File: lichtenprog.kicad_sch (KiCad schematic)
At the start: 54 parts, among them J1 USB_C_Receptacle_USB2.0, J2 IO_OUT, U1 AZ1117-ADJ, U2 MCP6L04x-xSL, U3 USBLC6-2SC6, U4 CP2102N-A01-GQFN28, U5 SN74LVC1T45DBV, U6 SN74LVC1T45DBV

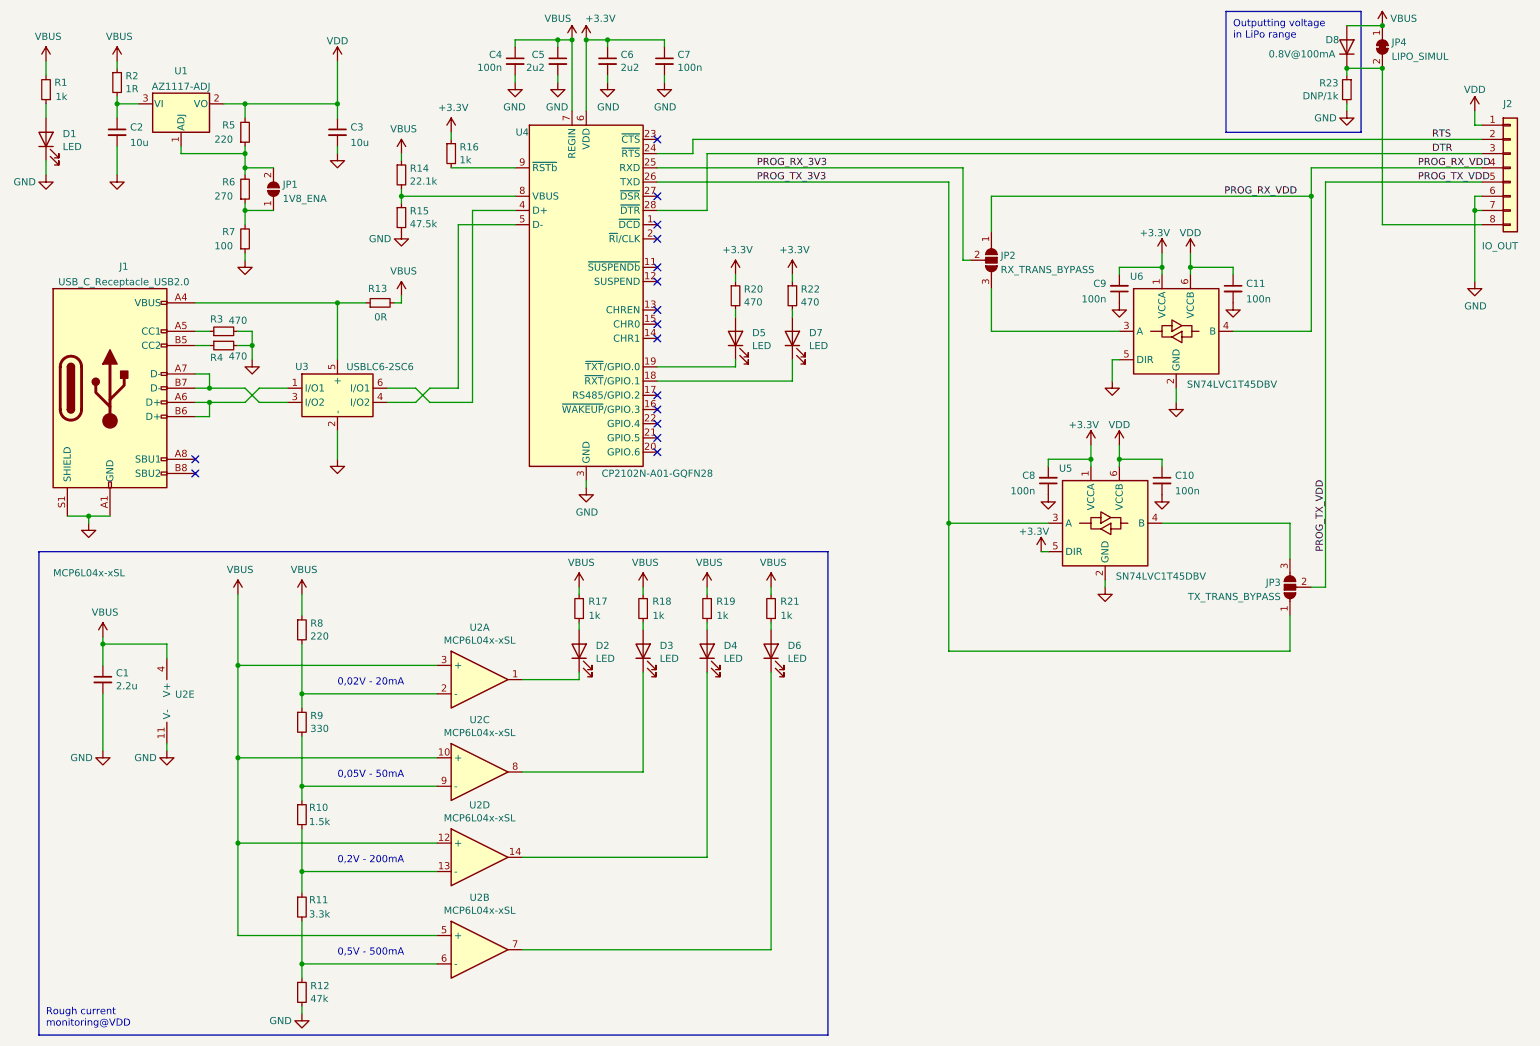
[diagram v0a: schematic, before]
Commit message: idk
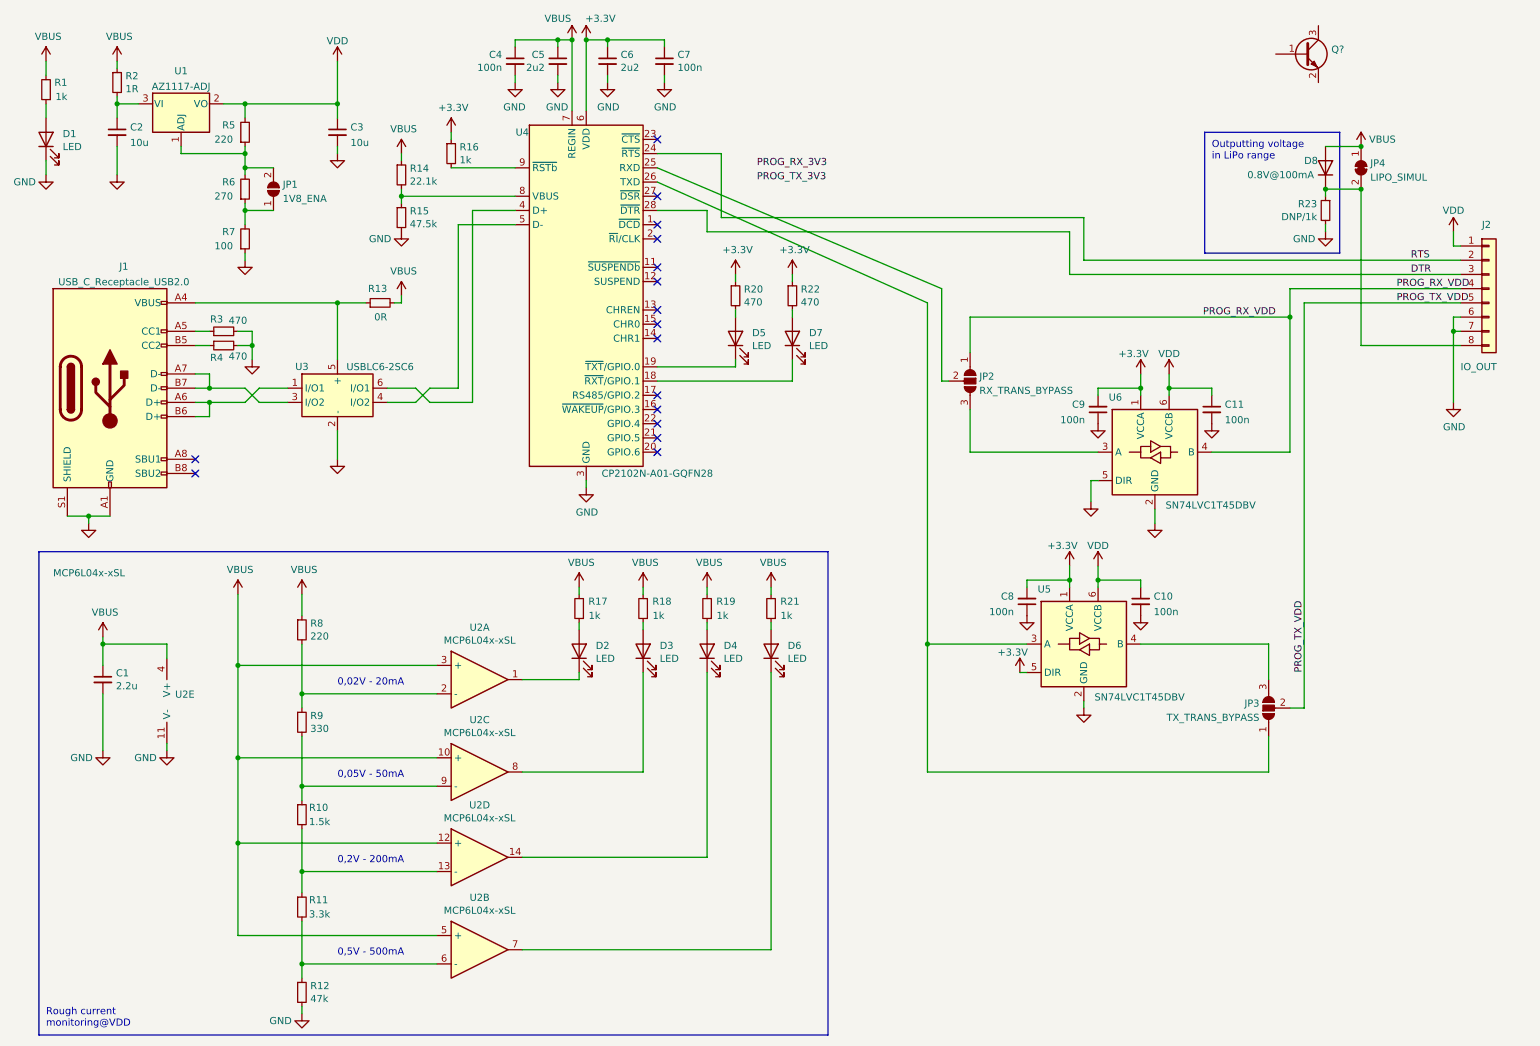
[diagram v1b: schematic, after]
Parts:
- added Q?: (no value), symbol Transistor_BJT:BC847
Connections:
- net PROG_RX_3V3: no longer JP2.2 (C), U4.25 (RXD)
- net PROG_TX_3V3: no longer JP3.1 (A), U4.26 (TXD), U5.3 (A)
- new net: JP2.2 (C), U4.25 (RXD)
- new net: JP3.1 (A), U4.26 (TXD), U5.3 (A)
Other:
- moved on the sheet: C10, C11, C8, C9, D8, J2, JP2, JP3, JP4, R23, U5, U6
